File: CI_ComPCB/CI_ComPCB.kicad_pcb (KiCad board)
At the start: 2 copper layers, 50 parts, among them IC301 TPS63020DSJR, J101 Conn_01x15_Female, J102 Conn_01x15_Female, J301 Connector_Conn_01x02_Male, J302 Connector_Conn_01x02_Male, J401 Connector_Conn_01x02_Male, J402 Connector_Conn_01x02_Male, J501 RJ45_LED_Shielded, J502 RJ45_LED_Shielded, Q201 Transistor_FET_IRF9540N, SW501 SW_DIP_x04, U101 ESP32s, U401 TPS54331

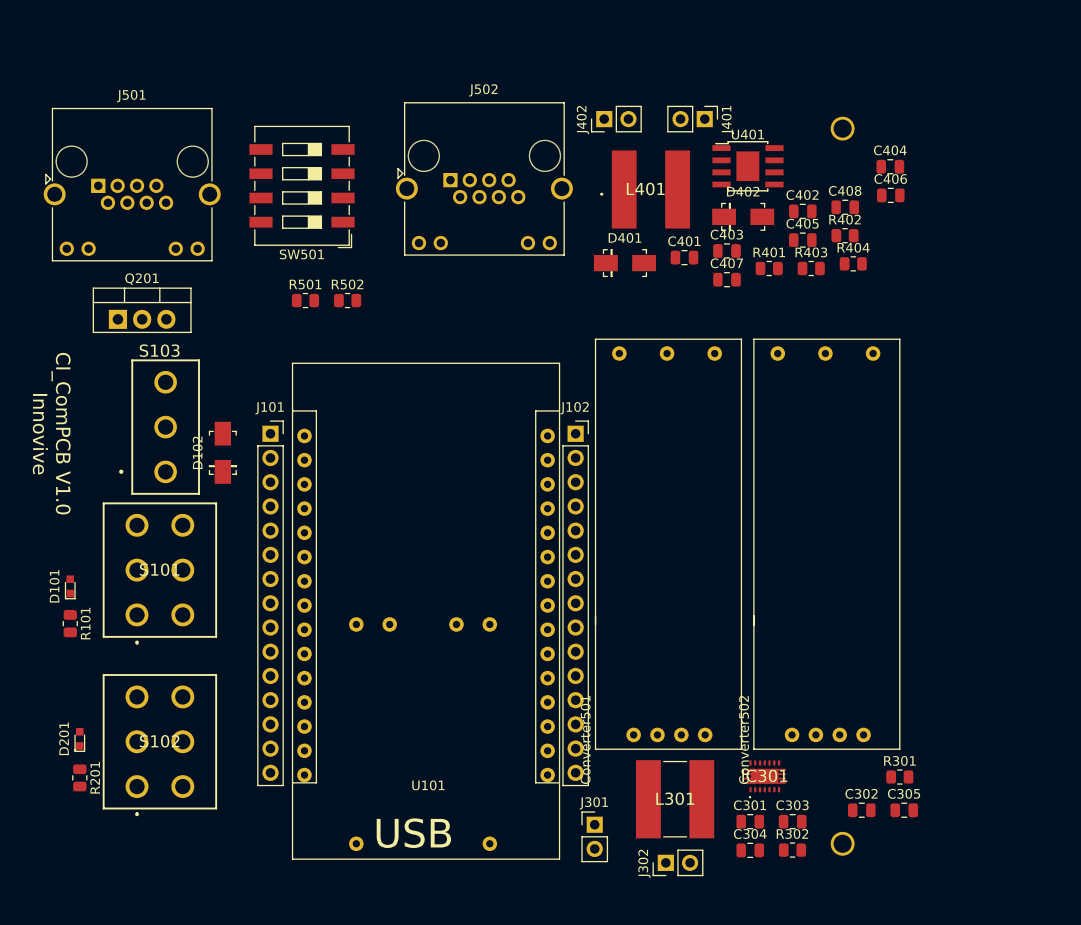
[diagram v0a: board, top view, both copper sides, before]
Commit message: V1.1 in progress
Completed Bom and schematic
still need to add routs and PCB layout
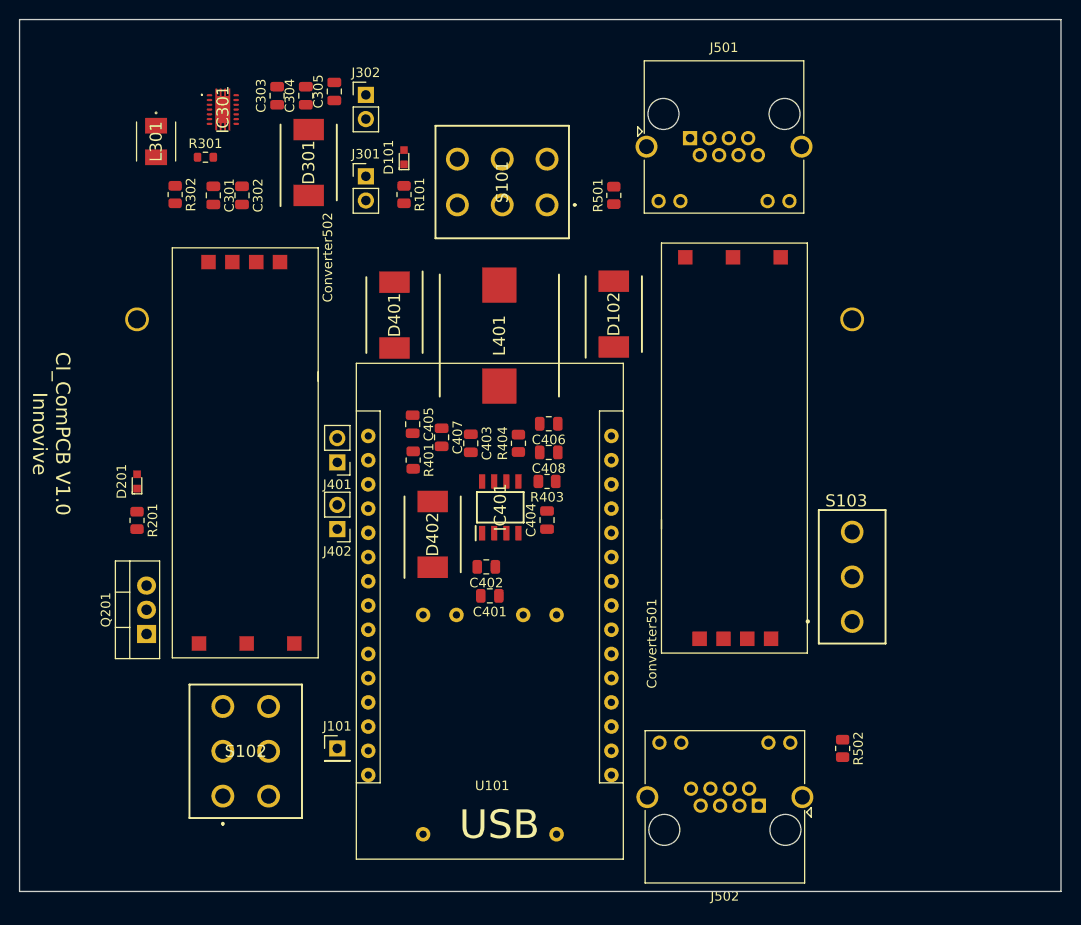
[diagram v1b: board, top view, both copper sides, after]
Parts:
- removed J102: Conn_01x15_Female, Connector_PinSocket_2.54mm:PinSocket_1x15_P2.54mm_Vertical
- removed R402: 0, Resistor_SMD:R_0805_2012Metric
- removed SW501: SW_DIP_x04, Button_Switch_SMD:SW_DIP_SPSTx04_Slide_9.78x12.34mm_W8.61mm_P2.54mm
- removed U401: TPS54331, Package_SO:TI_SO-PowerPAD-8
- added D301: SS34, SamacSys_Parts:DIOM8059X256N, F.Cu at (75.0, 86.5)
- added IC401: TPS54331DR, SamacSys_Parts:SOIC127P600X175-8N, F.Cu at (95.1, 122.7)
- D102, D401, D402: value B340A-13-F -> SS34; footprint digikey-footprints:DO-214AC -> SamacSys_Parts:DIOM8059X256N
- J101: value Conn_01x15_Female -> Conn_01x01_Male; footprint Connector_PinSocket_2.54mm:PinSocket_1x15_P2.54mm_Vertical -> Connector_PinHeader_2.54mm:PinHeader_1x01_P2.54mm_Vertical
- L301: value 1uH , 33mohm -> SPM4012T-1R0M-LR; footprint SamacSys_Parts:SRN8040R50Y -> SamacSys_Parts:SPM4010-4020
- L401: value SRN8040-100M -> RLF12560T-7R8N8R2; footprint SamacSys_Parts:SRN8040100M -> SamacSys_Parts:INDPM128125X600N
- R301: footprint Resistor_SMD:R_0805_2012Metric -> Resistor_SMD:R_0603_1608Metric
- R302: value 135k -> 130k
- R401: value 49.9k -> 56.2k
- R404: value 1.91k -> 1.78k
- moved R301 97.6 mm to (64.2, 86.0)
- moved C305 96.2 mm to (77.7, 79.1), turned to 90 degrees
- moved R302 94.4 mm to (61.0, 89.9), turned to 270 degrees
- moved C303 93.4 mm to (71.7, 79.5), turned to 90 degrees
- moved C304 91.8 mm to (74.7, 79.5), turned to 90 degrees
- moved C302 91.6 mm to (68.0, 90.0), turned to 270 degrees
- moved IC301 90.1 mm to (66.0, 81.0), turned to 270 degrees
- moved L301 87.9 mm to (59.0, 84.3), turned to 270 degrees
- moved C301 86.5 mm to (65.0, 90.0), turned to 270 degrees
- moved J302 86.5 mm to (81.0, 79.5), turned to 0 degrees
- moved S103 73.7 mm to (132.0, 130.0)
- moved J502 73.1 mm to (122.2, 154.0), turned to 180 degrees
- moved J301 72.1 mm to (81.0, 88.0)
- moved R502 70.0 mm to (131.0, 148.0), turned to 270 degrees
- moved Converter502 69.7 mm to (76.0, 95.5), turned to 270 degrees
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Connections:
- J101 pad 1: Net-(J101-Pad1) -> GND
- J301 pad 1: Net-(C301-Pad1) -> Net-(D301-Pad1)
- J402 pad 2: Net-(D402-PadK) -> Net-(D402-Pad1)
- J502 pad 3: Net-(J502-Pad3) -> Net-(J501-Pad3)
- J502 pad 4: Net-(J502-Pad4) -> Net-(J501-Pad4)
- J502 pad 5: Net-(J502-Pad5) -> Net-(J501-Pad5)
- J502 pad 6: Net-(J502-Pad6) -> Net-(J501-Pad6)
- R403 pad 1: Net-(R402-Pad2) -> Net-(C406-Pad1)
- S101 pad 6: Net-(D102-PadK) -> Net-(D102-Pad1)
- U101 pad D12: Net-(J101-Pad12) -> Net-(U101-PadD12)
- U101 pad D13: Net-(J101-Pad13) -> Net-(U101-PadD13)
- U101 pad D14: Net-(J101-Pad11) -> Net-(U101-PadD14)
- U101 pad D25: Net-(J101-Pad8) -> Net-(U101-PadD25)
- U101 pad D26: Net-(J101-Pad9) -> Net-(U101-PadD26)
- U101 pad D27: Net-(J101-Pad10) -> Net-(U101-PadD27)
- U101 pad D32: Net-(J101-Pad6) -> Net-(U101-PadD32)
- U101 pad D33: Net-(J101-Pad7) -> Net-(U101-PadD33)
- U101 pad D34: Net-(J101-Pad4) -> Net-(U101-PadD34)
- U101 pad D35: Net-(J101-Pad5) -> Net-(U101-PadD35)
- U101 pad EN: Net-(J101-Pad1) -> Net-(U101-PadEN)
- U101 pad VN: Net-(J101-Pad3) -> Net-(U101-PadVN)
- U101 pad VP: Net-(J101-Pad2) -> Net-(U101-PadVP)
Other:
- board outline added: 109.2 x 91.4 mm
